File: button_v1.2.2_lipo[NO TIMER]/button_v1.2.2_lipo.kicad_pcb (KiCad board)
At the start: 2 copper layers, 21 x 41.7 mm, 17 parts, among them J1 Conn_01x05_Female, SW1 SW_Push, SW2 SW_Push, U2 AP2112K-3.3, X1 ESP-12E

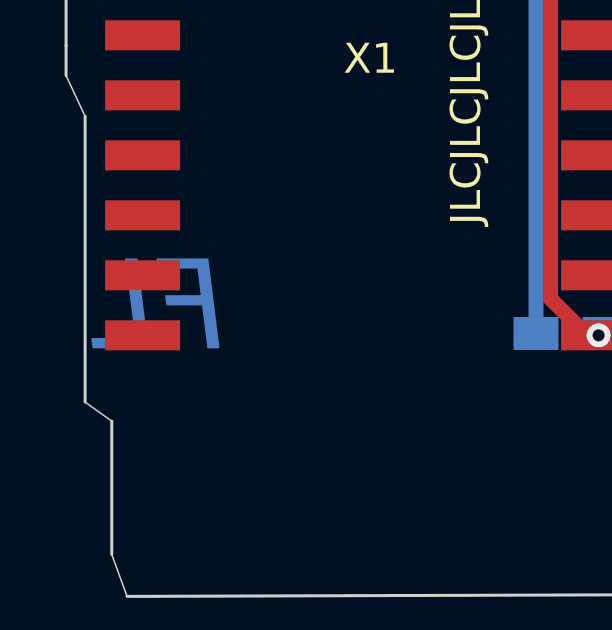
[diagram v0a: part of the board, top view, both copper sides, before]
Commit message: 23.02 00:38
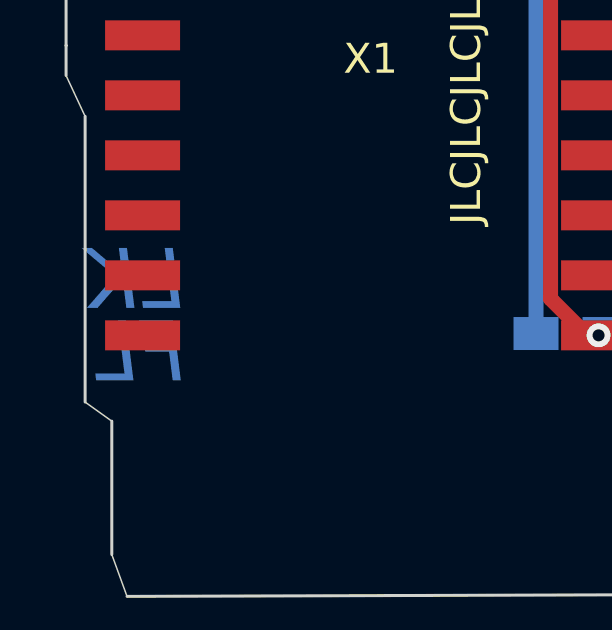
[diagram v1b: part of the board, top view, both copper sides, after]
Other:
- board text added: "LK"
